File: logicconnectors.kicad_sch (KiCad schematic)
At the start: 26 parts, among them J1 USBC Socket, J2 CANConn, J3 HallConn, J4 Conn_ARM_JTAG_SWD_20, J5 UART2, J6 InputConn, J7 UART, J8 DriverBoardConn, U2 USBLC6-2P6, U3 TJA1051T-3

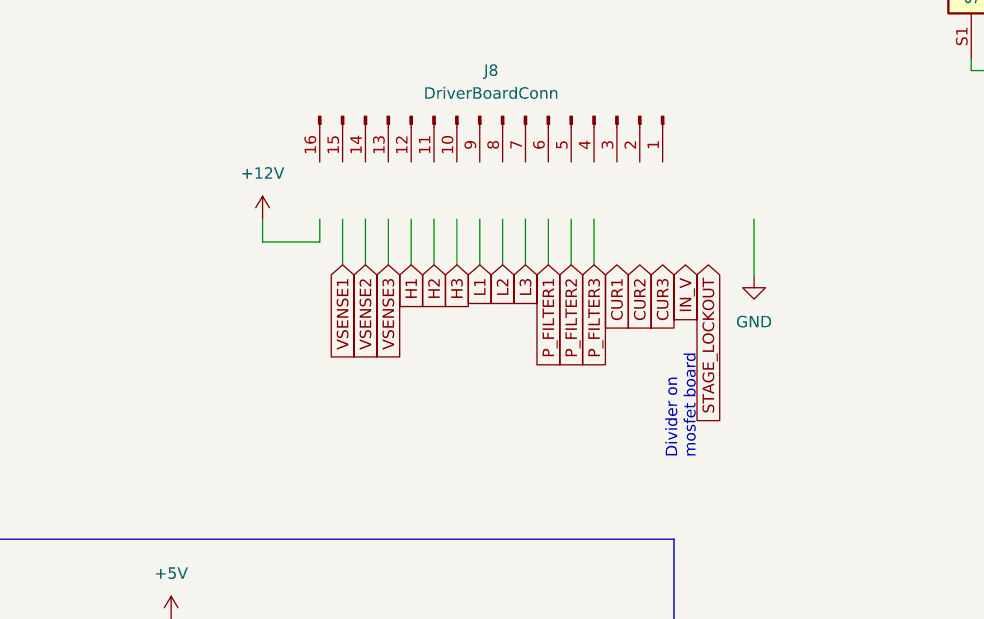
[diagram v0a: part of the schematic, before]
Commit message: drivers
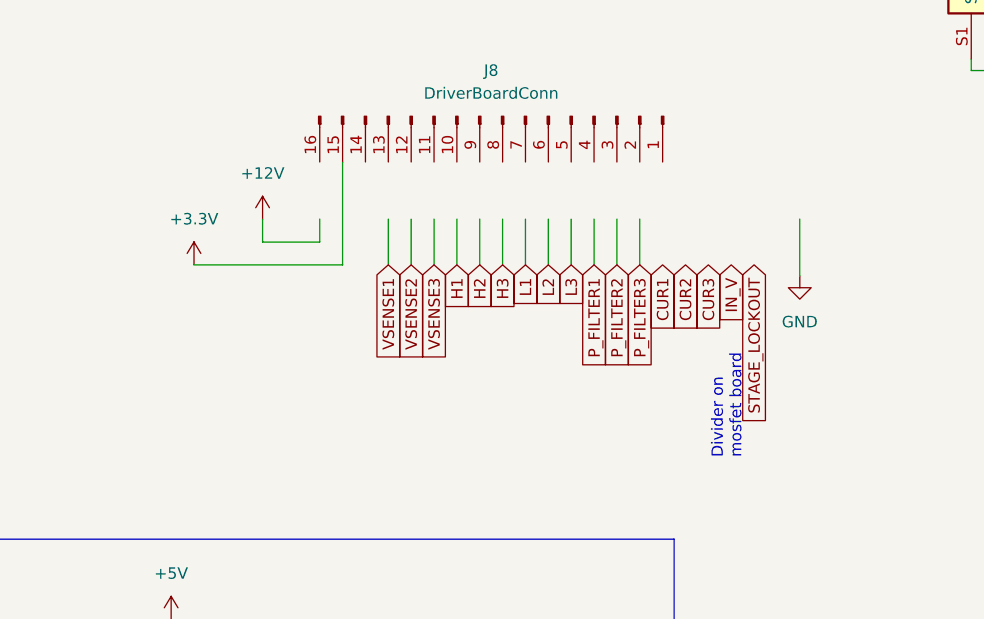
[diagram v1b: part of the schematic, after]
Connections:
- net +3.3V: now also J8.15 (Pin_15)

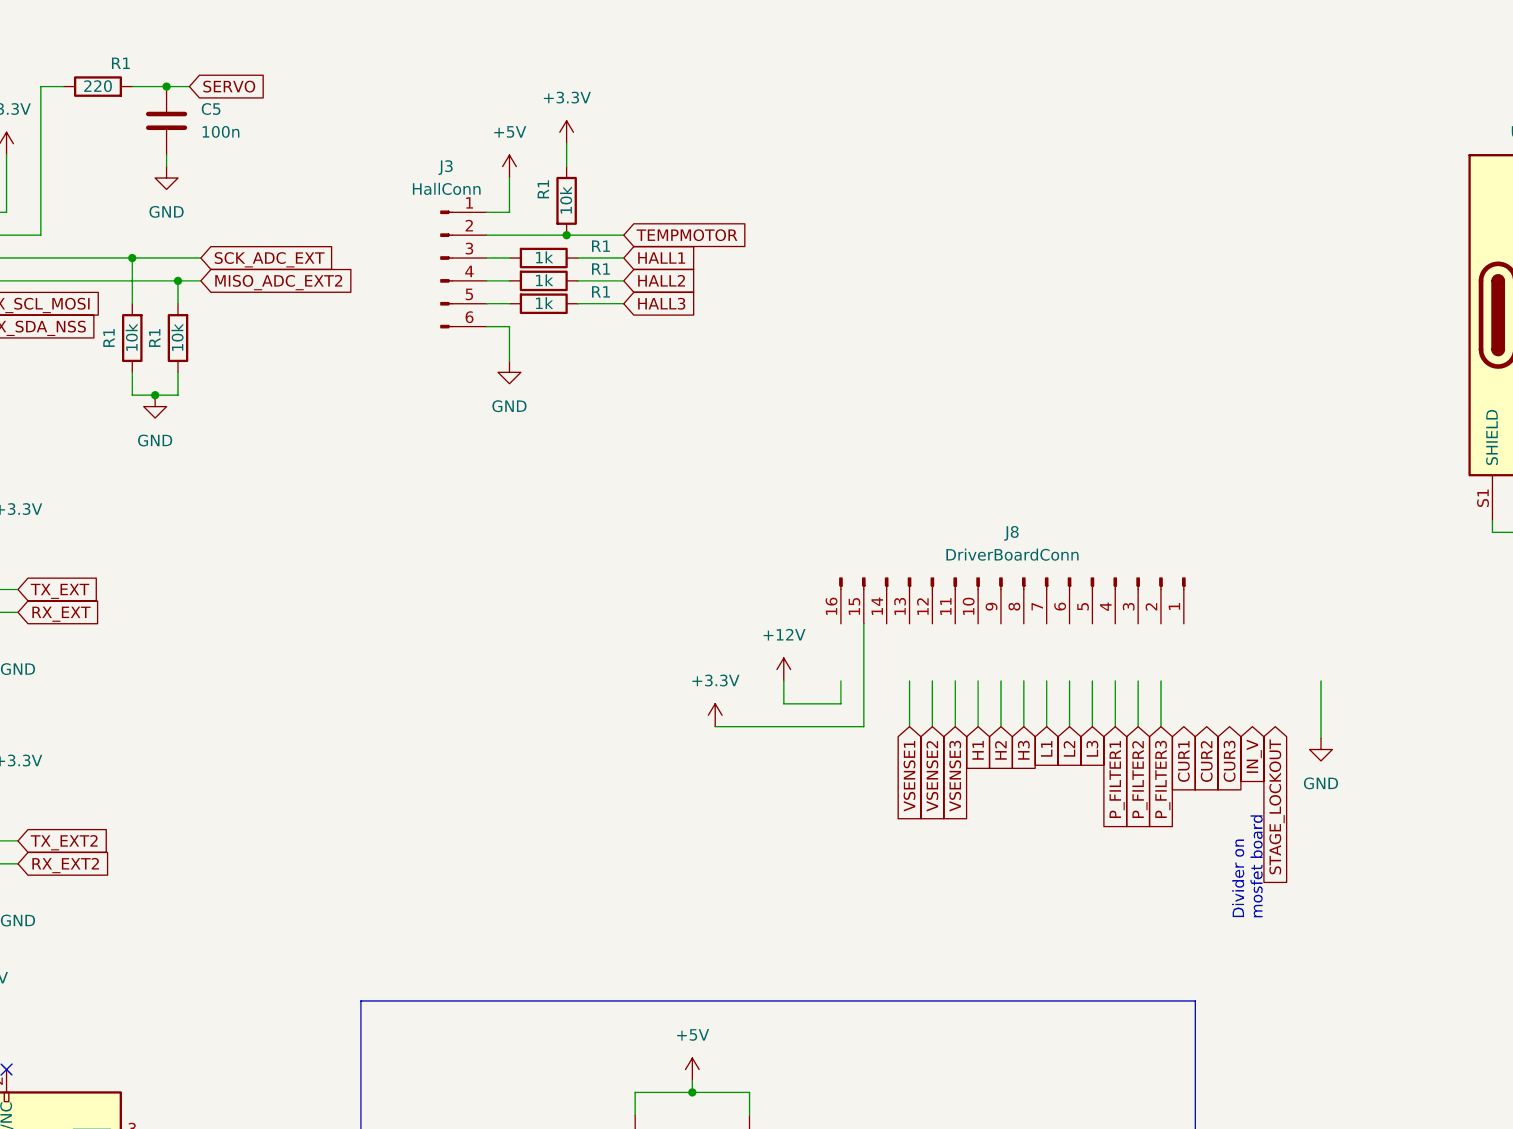
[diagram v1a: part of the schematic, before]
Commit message: initial
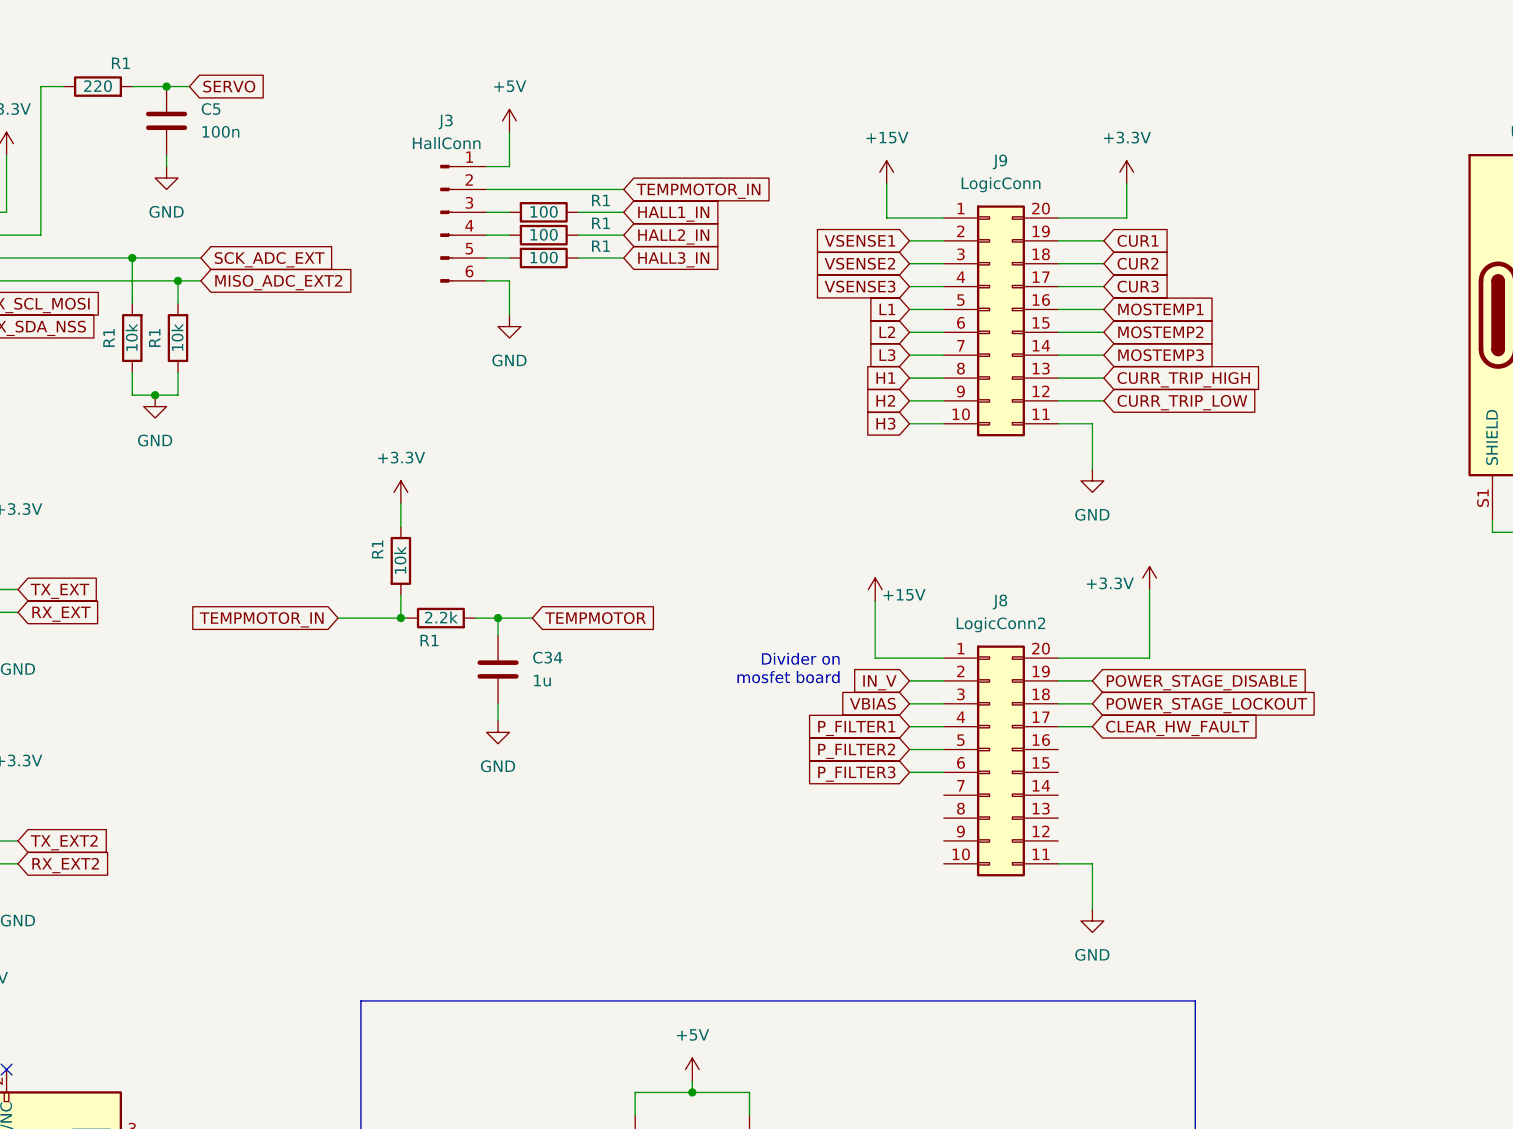
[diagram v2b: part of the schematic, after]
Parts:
- removed J8: DriverBoardConn, symbol Connector:Conn_01x16_Pin
- added C34: 1u, symbol Device:C
- added J8: LogicConn2, symbol Connector_Generic:Conn_02x10_Counter_Clockwise
- added J9: LogicConn, symbol Connector_Generic:Conn_02x10_Counter_Clockwise
- added R1: 2.2k, symbol Device:R
- R1: value 1k -> 100
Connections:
- net +3.3V: now also J8.20 (Pin_20), J9.20 (Pin_20)
- net CUR1: now also J9.19 (Pin_19)
- net CUR2: now also J9.18 (Pin_18)
- net CUR3: now also J9.17 (Pin_17)
- net GND: now also C34.2, J8.11 (Pin_11), J9.11 (Pin_11)
- net H1: now also J9.8 (Pin_8)
- net H2: now also J9.9 (Pin_9)
- net H3: now also J9.10 (Pin_10)
- net IN_V: now also J8.2 (Pin_2)
- net L1: now also J9.5 (Pin_5)
- net L2: now also J9.6 (Pin_6)
- net L3: now also J9.7 (Pin_7)
- net P_FILTER1: now also J8.4 (Pin_4)
- net P_FILTER2: now also J8.5 (Pin_5)
- net P_FILTER3: now also J8.6 (Pin_6)
- net TEMPMOTOR: now also C34.1, R1.2; no longer J3.2 (Pin_2), R1.2
- net VSENSE1: now also J9.2 (Pin_2)
- net VSENSE2: now also J9.3 (Pin_3)
- net VSENSE3: now also J9.4 (Pin_4)
- net HALL1 renamed HALL1_IN
- net HALL2 renamed HALL2_IN
- net HALL3 renamed HALL3_IN
- new net +15V: J8.1 (Pin_1), J9.1 (Pin_1)
- new net CLEAR_HW_FAULT: J8.17 (Pin_17)
- new net CURR_TRIP_HIGH: J9.13 (Pin_13)
- new net CURR_TRIP_LOW: J9.12 (Pin_12)
- new net MOSTEMP1: J9.16 (Pin_16)
- new net MOSTEMP2: J9.15 (Pin_15)
- new net MOSTEMP3: J9.14 (Pin_14)
- new net POWER_STAGE_DISABLE: J8.19 (Pin_19)
- new net POWER_STAGE_LOCKOUT: J8.18 (Pin_18)
- new net TEMPMOTOR_IN: J3.2 (Pin_2), R1.1, R1.2
- new net VBIAS: J8.3 (Pin_3)
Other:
- moved on the sheet: J3, R1

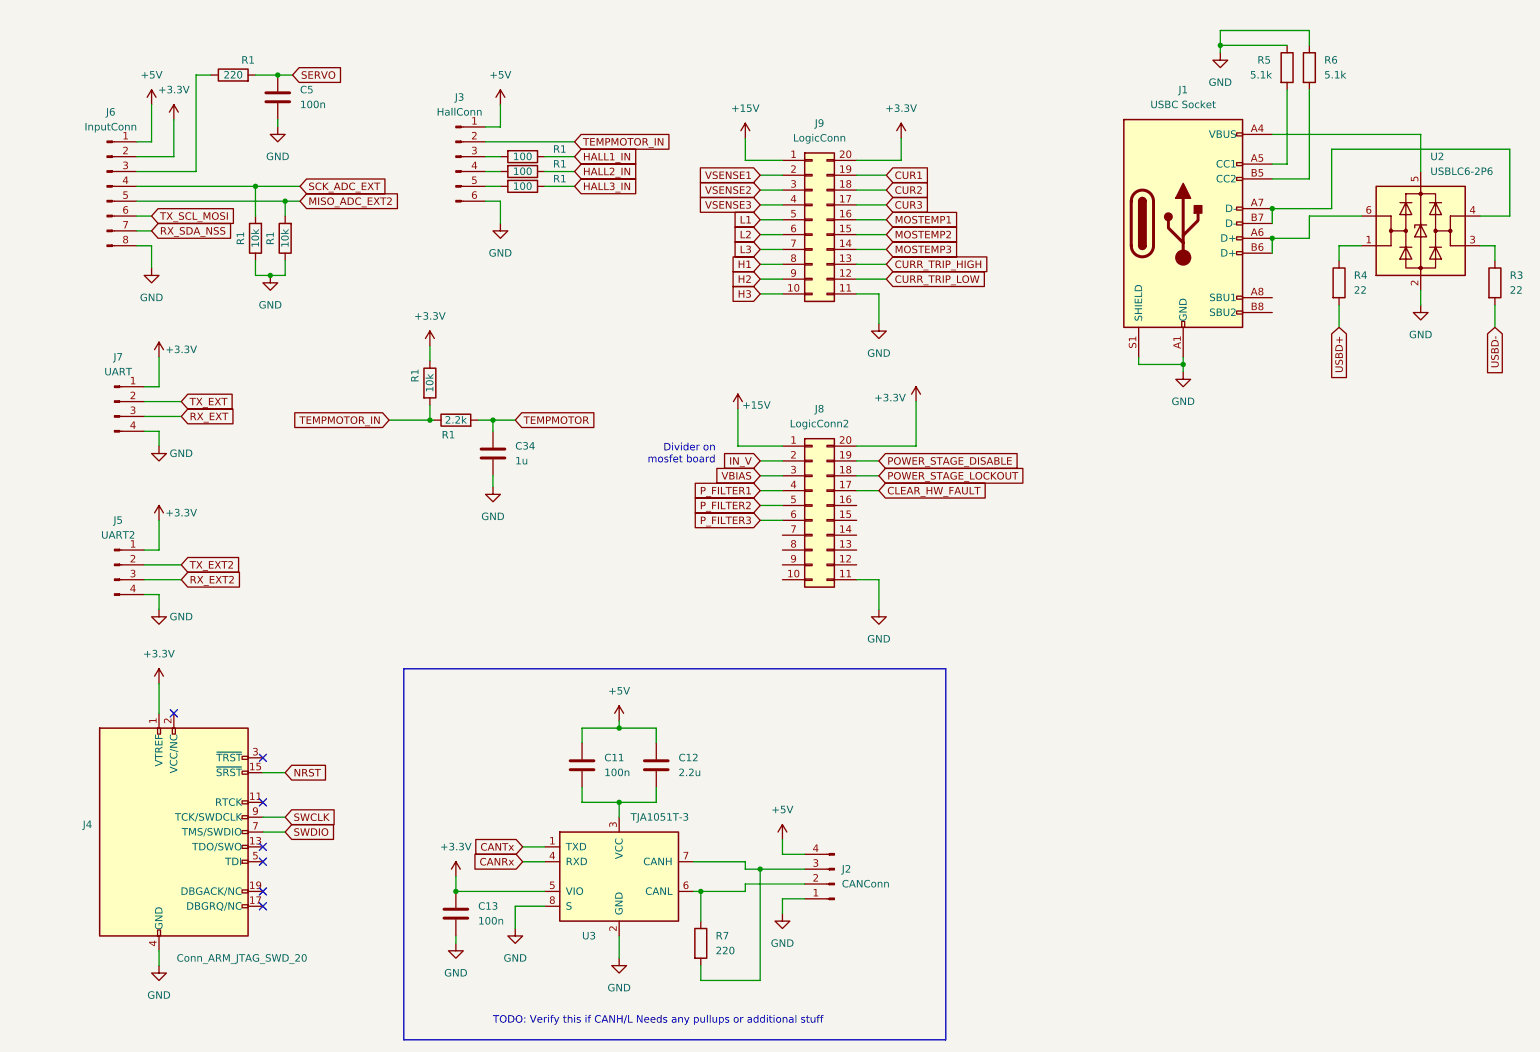
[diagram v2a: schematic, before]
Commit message: initial
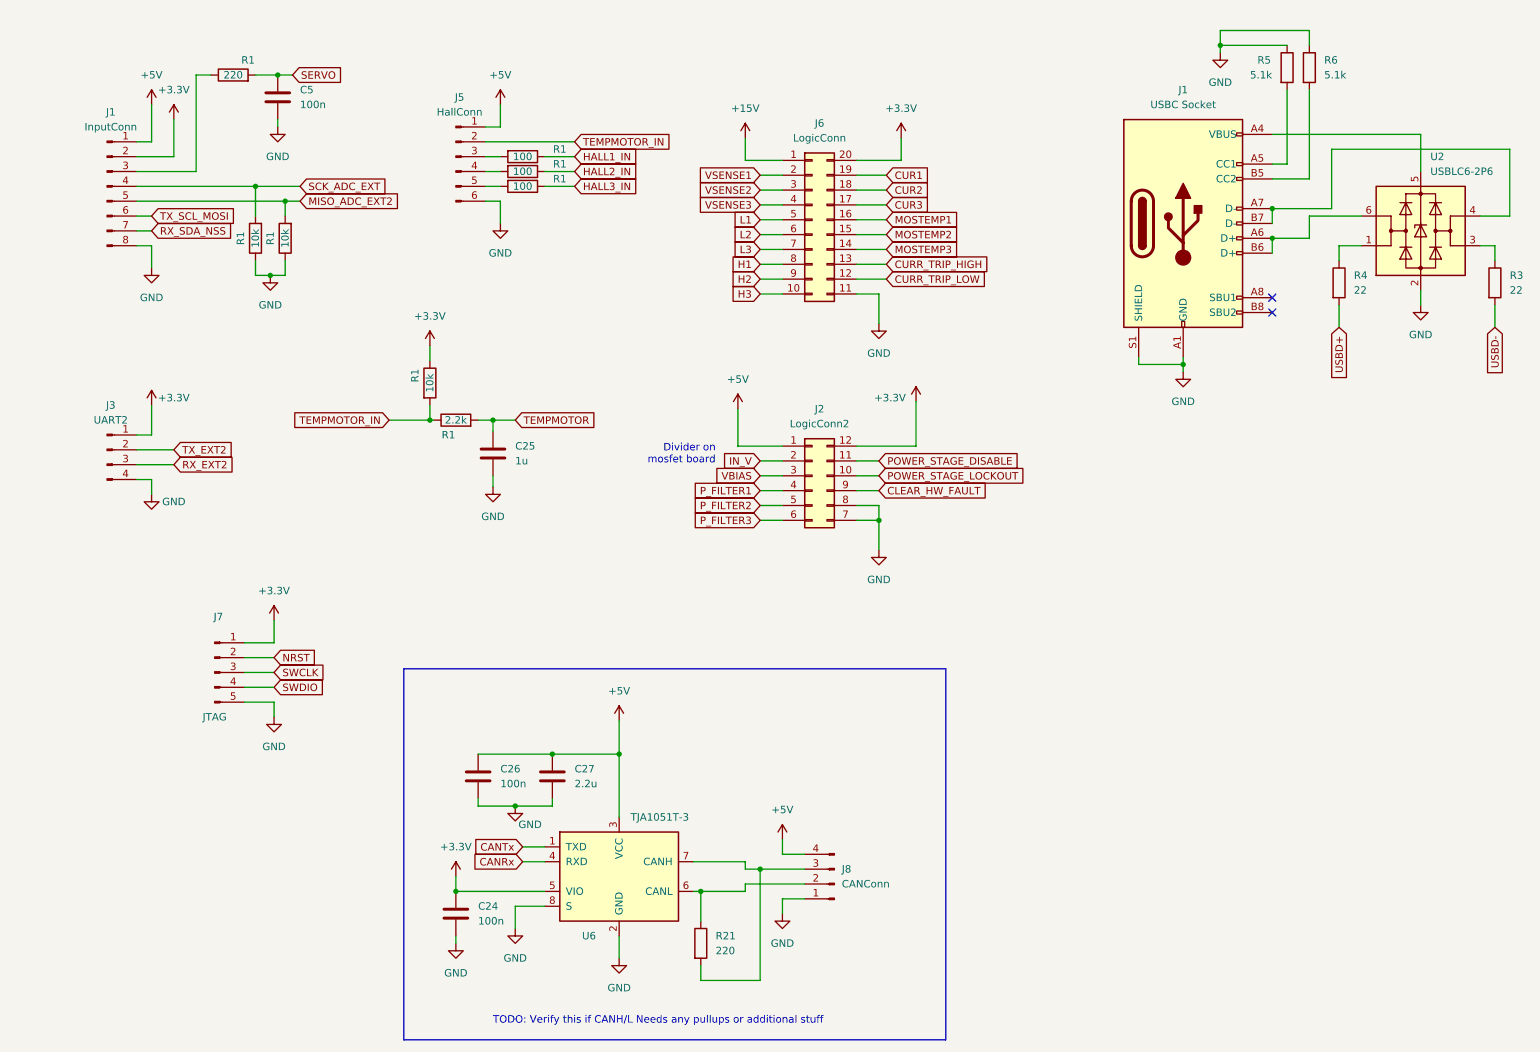
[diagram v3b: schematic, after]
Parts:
- removed J4: Conn_ARM_JTAG_SWD_20, symbol Connector:Conn_ARM_JTAG_SWD_20
- removed J7: UART, symbol Connector:Conn_01x04_Pin
- removed J8: LogicConn2, symbol Connector_Generic:Conn_02x10_Counter_Clockwise
- added J2: LogicConn2, Connector_PinHeader_2.54mm:PinHeader_2x06_P2.54mm_Vertical, symbol Connector_Generic:Conn_02x06_Counter_Clockwise
- added J7: JTAG, Connector_PinHeader_2.54mm:PinHeader_1x05_P2.54mm_Vertical, symbol Connector:Conn_01x05_Pin
- C24: renamed from C13; footprint (none) -> Capacitor_SMD:C_0805_2012Metric
- C25: renamed from C34; footprint (none) -> Capacitor_SMD:C_0805_2012Metric
- C26: renamed from C11; footprint (none) -> Capacitor_SMD:C_0805_2012Metric
- C27: renamed from C12; footprint (none) -> Capacitor_SMD:C_0805_2012Metric
- C5: footprint (none) -> Capacitor_SMD:C_0805_2012Metric
- J1: footprint (none) -> Connector_USB:USB_C_Receptacle_GCT_USB4105-xx-A_16P_TopMnt_Horizontal
- J1: renamed from J6; footprint (none) -> Connector_PinHeader_2.54mm:PinHeader_1x08_P2.54mm_Horizontal
- J3: renamed from J5; footprint (none) -> Connector_PinHeader_2.54mm:PinHeader_1x04_P2.54mm_Horizontal
- J5: renamed from J3; footprint (none) -> Connector_PinHeader_2.54mm:PinHeader_1x06_P2.54mm_Horizontal
- J6: renamed from J9; footprint (none) -> Connector_PinHeader_2.54mm:PinHeader_2x10_P2.54mm_Vertical
- J8: renamed from J2; footprint (none) -> Connector_PinHeader_2.54mm:PinHeader_1x04_P2.54mm_Horizontal
- R1, R3, R4, R5, R6: footprint (none) -> Resistor_SMD:R_0805_2012Metric
- R21: renamed from R7; footprint (none) -> Resistor_SMD:R_0805_2012Metric
- renumbered U3 to U6
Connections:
- net +3.3V: now also J2.12 (Pin_12), J7.1 (Pin_1)
- net +5V: now also U6.3 (VCC), J2.1 (Pin_1)
- net CLEAR_HW_FAULT: now also J2.9 (Pin_9)
- net GND: now also C26.2, C27.2, J2.7 (Pin_7), J2.8 (Pin_8), J7.5 (Pin_5)
- net IN_V: now also J2.2 (Pin_2)
- net NRST: now also J7.2 (Pin_2)
- net POWER_STAGE_DISABLE: now also J2.11 (Pin_11)
- net POWER_STAGE_LOCKOUT: now also J2.10 (Pin_10)
- net P_FILTER1: now also J2.4 (Pin_4)
- net P_FILTER2: now also J2.5 (Pin_5)
- net P_FILTER3: now also J2.6 (Pin_6)
- net SWCLK: now also J7.3 (Pin_3)
- net SWDIO: now also J7.4 (Pin_4)
- net VBIAS: now also J2.3 (Pin_3)
- no-connect marks 7 -> 2
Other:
- moved on the sheet: C26, C27, J3
